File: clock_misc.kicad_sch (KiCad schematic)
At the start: 12 parts, among them Y1 Osc60MHz

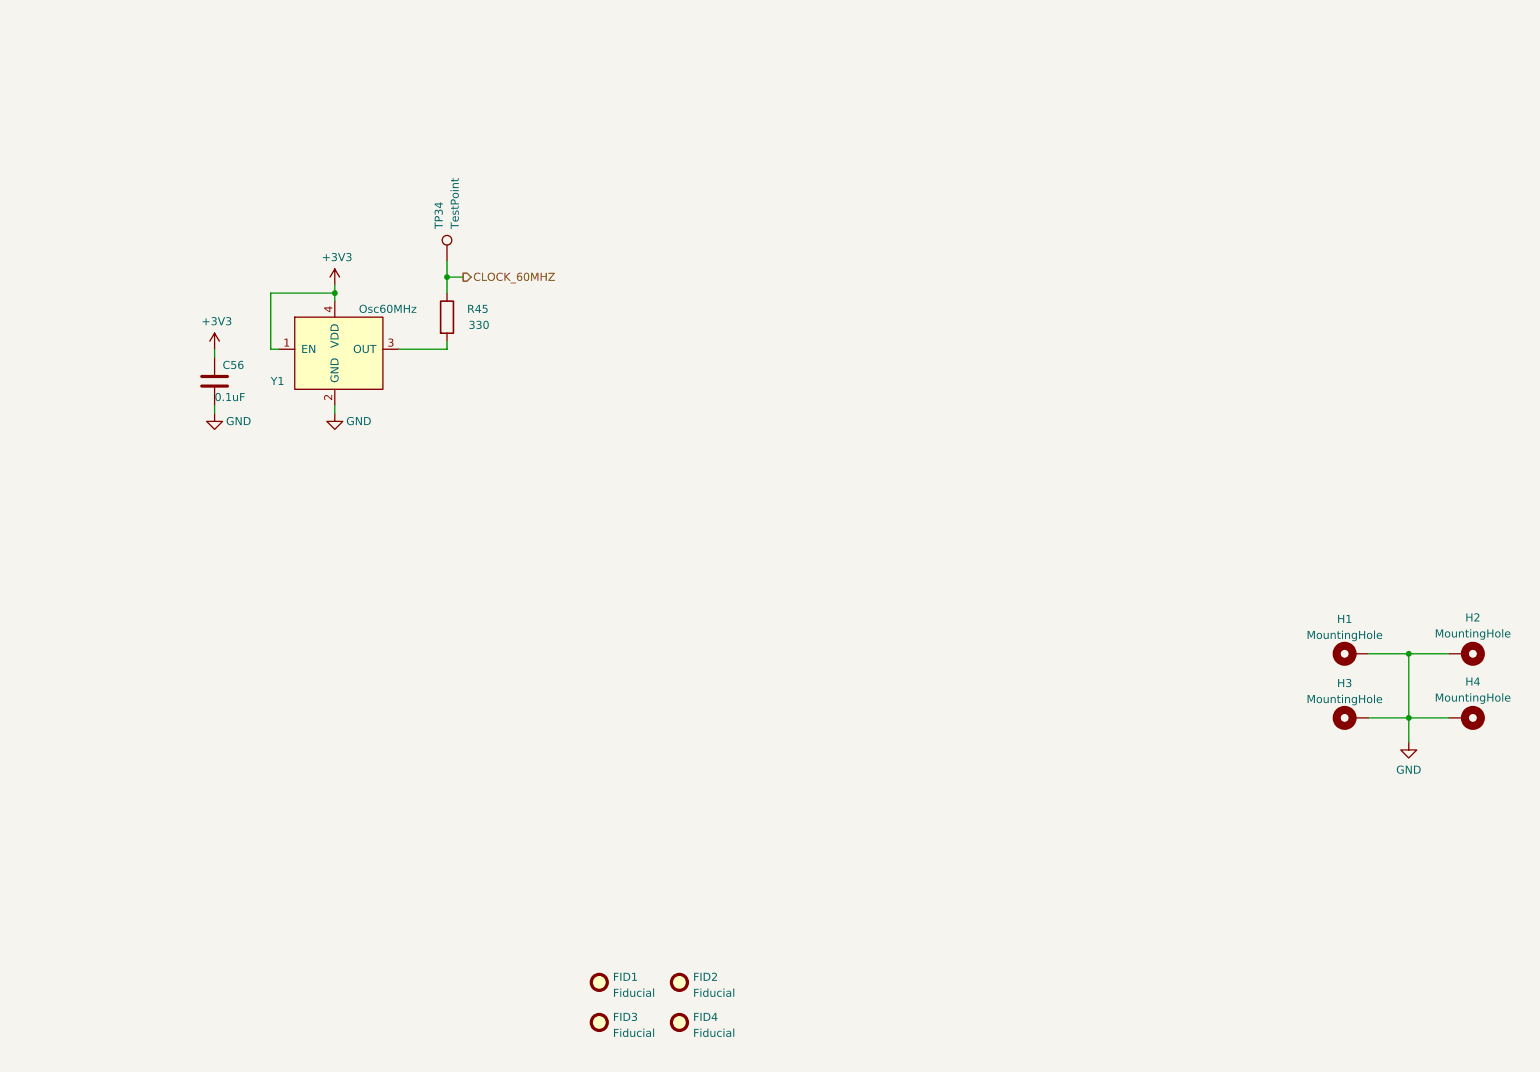
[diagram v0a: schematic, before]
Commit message: schematic wip
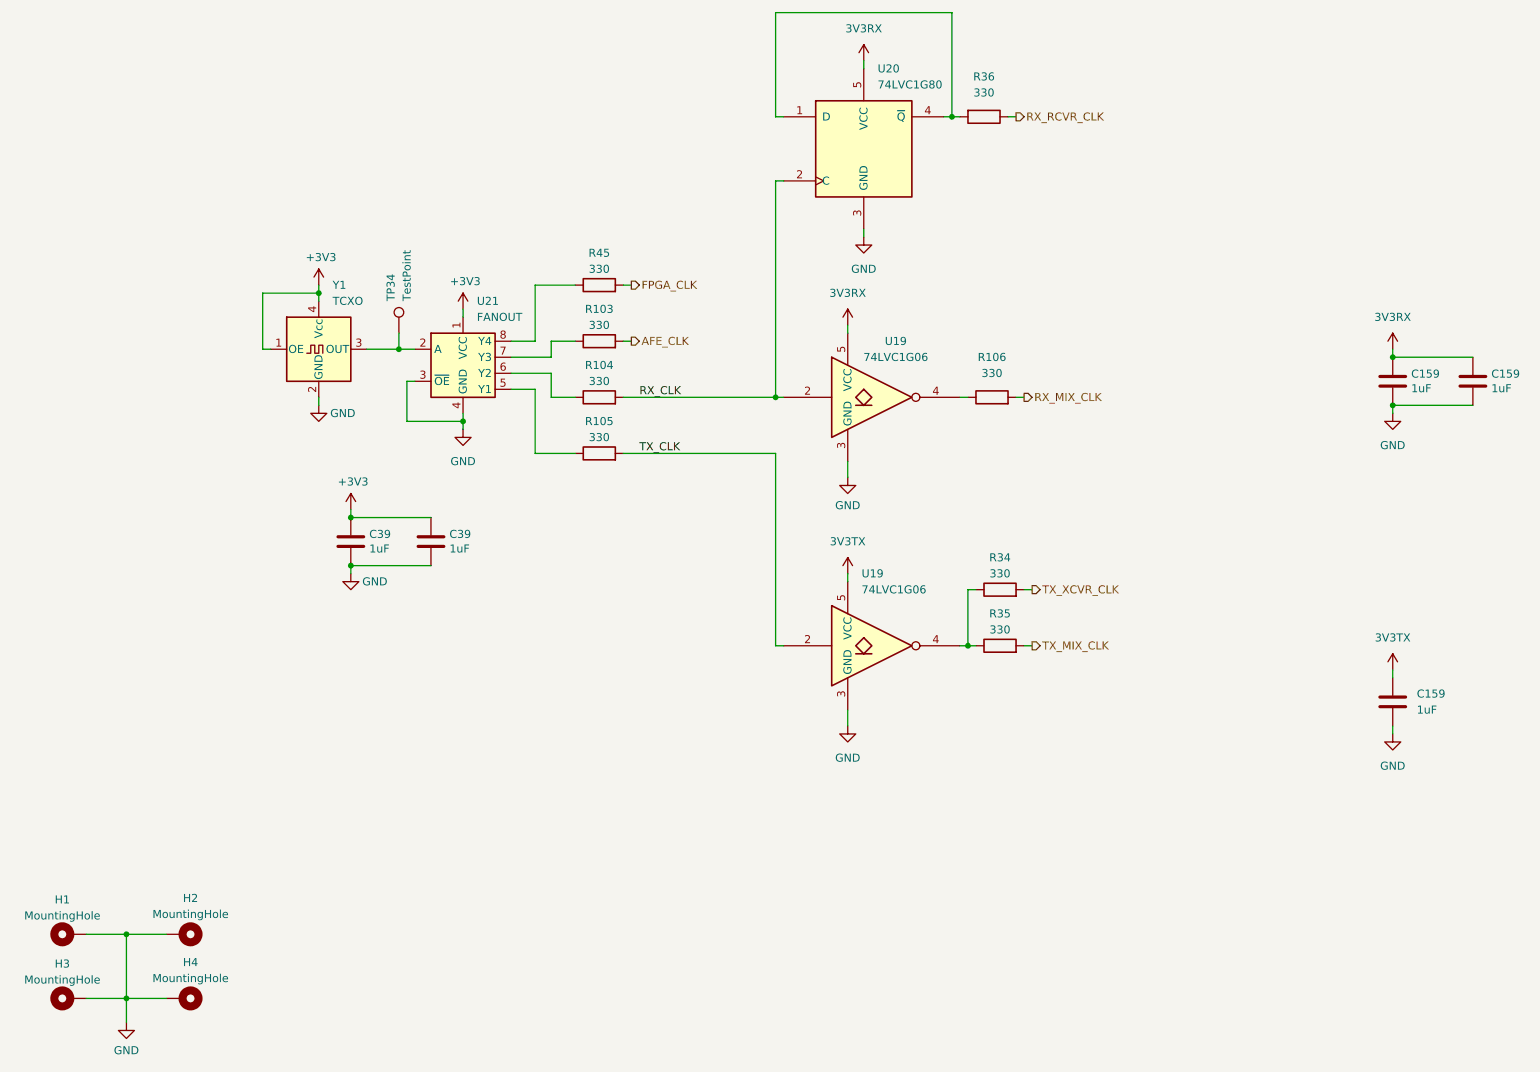
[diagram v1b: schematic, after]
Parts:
- removed C56: 0.1uF, Capacitor_SMD:C_0402_1005Metric, symbol Device:C
- removed FID1, FID2, FID3, FID4: Fiducial, Fiducial:Fiducial_0.5mm_Mask1mm, symbol Mechanical:Fiducial
- removed Y1: Osc60MHz, Crystal:Crystal_SMD_3225-4Pin_3.2x2.5mm, symbol support_hardware:DSC60xx
- added C159 (x3), C39 (x2): 1uF, Capacitor_SMD:C_0402_1005Metric, symbol Device:C
- added R103, R104, R105, R106, R34, R35, R36: 330, Resistor_SMD:R_0402_1005Metric, symbol Device:R
- added U19 (x2): 74LVC1G06, Package_TO_SOT_SMD:SOT-353_SC-70-5, symbol 74xGxx:74LVC1G06
- added U20: 74LVC1G80, Package_TO_SOT_SMD:SOT-353_SC-70-5, symbol 74xGxx:74AUP1G80
- added U21: FANOUT, symbol support_hardware:74AVC9112
- added Y1: TCXO, Oscillator:Oscillator_SMD_Kyocera_KC2520Z-4Pin_2.5x2.0mm, symbol Oscillator:SG-210SCD
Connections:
- net +3V3: now also C39.1, C39.1, U21.1 (VCC), Y1.1 (OE), Y1.4 (Vcc)
- net GND: now also C159.2, C159.2, C159.2, C39.2, C39.2, U19.3 (GND), U19.3 (GND), U20.3 (GND), U21.3 (~{OE}), U21.4 (GND), Y1.2 (GND)
- net FPGA_CLK: now reaches R45.2
- net CLOCK_60MHZ: no longer names the net of TP34.1
- net CLOCK_60MHZ: now also U21.2 (A), Y1.3 (OUT); no longer R45.1
- new net: R105.1, U21.5 (Y1)
- new net: R104.1, U21.6 (Y2)
- new net: R103.1, U21.7 (Y3)
- new net: R45.1, U21.8 (Y4)
- new net: R36.2, U20.1 (D), U20.4 (~{Q})
- new net: R34.1, R35.1, U19.4
- new net: R106.1, U19.4
- new net 3V3RX: C159.1, C159.1, U19.5 (VCC), U20.5 (VCC)
- new net 3V3TX: C159.1, U19.5 (VCC)
- new net AFE_CLK: R103.2
- new net RX_CLK: R104.2, U19.2, U20.2 (C)
- new net RX_MIX_CLK: R106.2
- new net RX_RCVR_CLK: R36.1
- new net TX_CLK: R105.2, U19.2
- new net TX_MIX_CLK: R35.2
- new net TX_XCVR_CLK: R34.2
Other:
- moved on the sheet: H1, H2, H3, H4, R45, TP34
